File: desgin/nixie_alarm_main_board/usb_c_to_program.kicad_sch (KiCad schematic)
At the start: 3 parts, among them J3 USB_C_Receptacle_USB2.0_16P

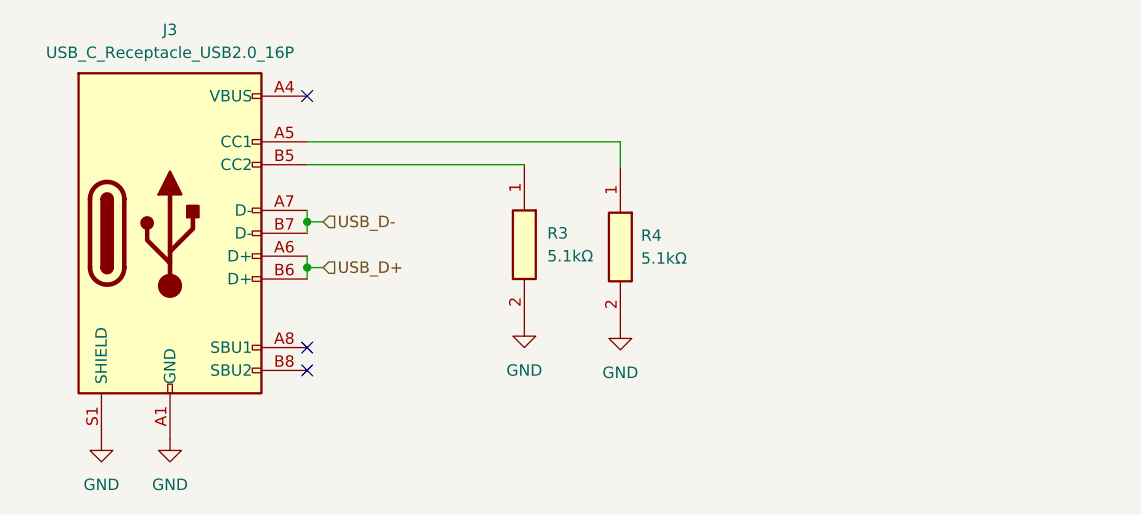
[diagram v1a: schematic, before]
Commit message: tvs protection try
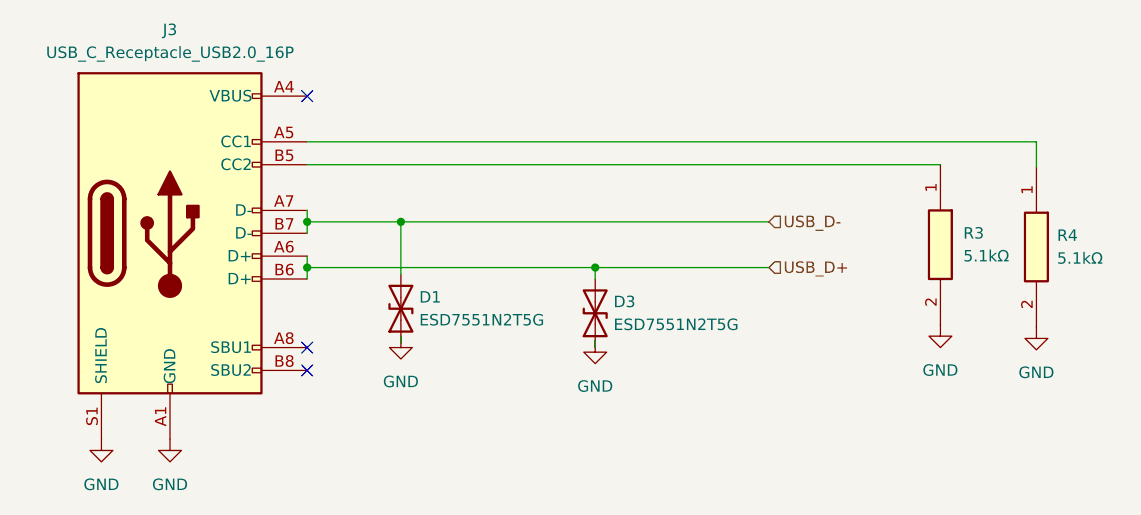
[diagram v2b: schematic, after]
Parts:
- added D1, D3: ESD7551N2T5G, ESD7551N2T5G, symbol Device:D_TVS
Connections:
- net GND: now also D1.1 (A1), D3.1 (A1)
- net USB_D+: now also D3.2 (A2)
- net USB_D-: now also D1.2 (A2)
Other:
- moved on the sheet: R3, R4
